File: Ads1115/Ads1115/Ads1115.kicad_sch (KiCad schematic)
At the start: 5 parts, among them U1 ADS1115IDGS

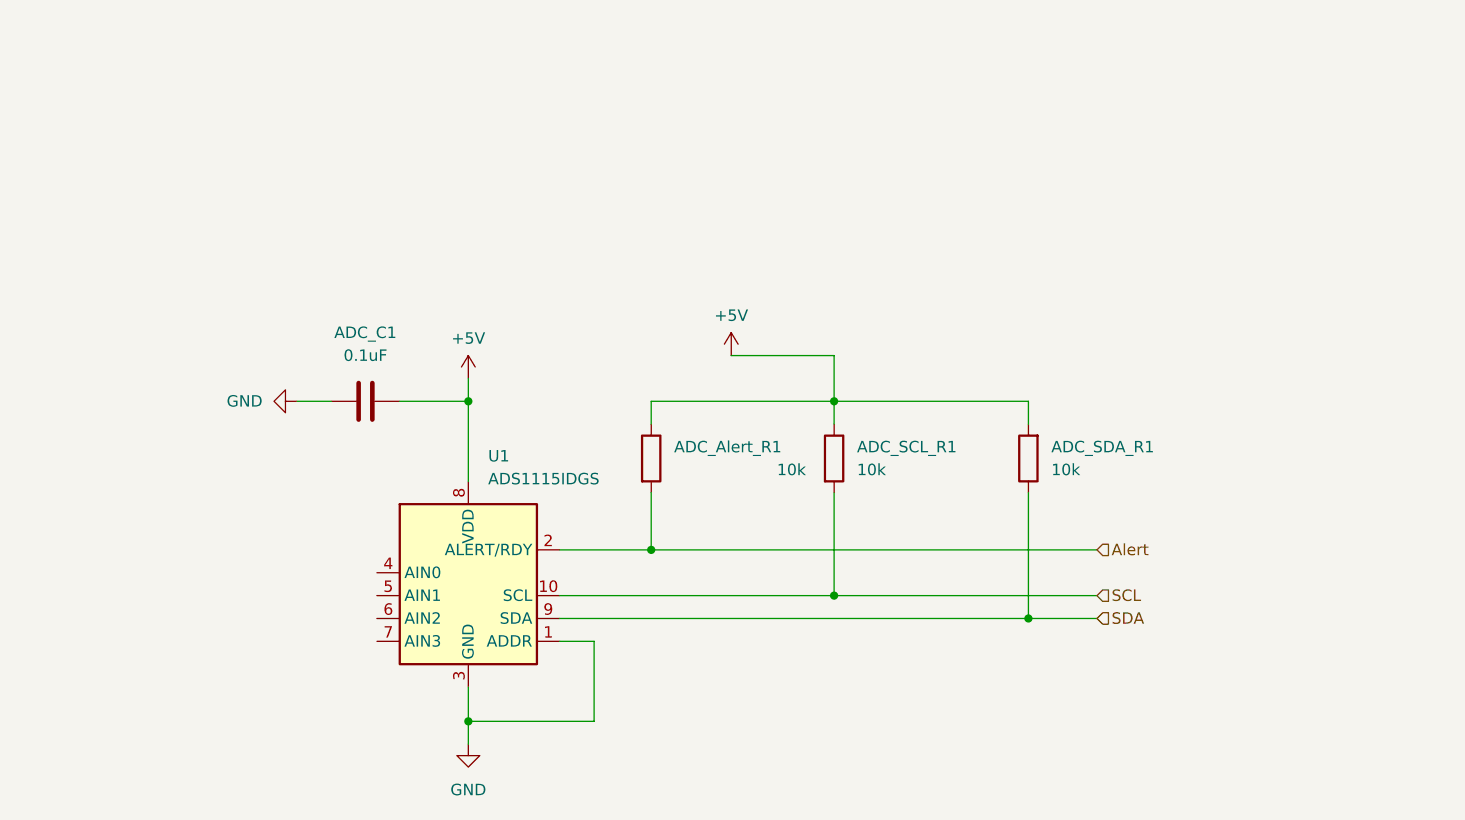
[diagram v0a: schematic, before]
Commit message: updates ads1115 and ads 1248
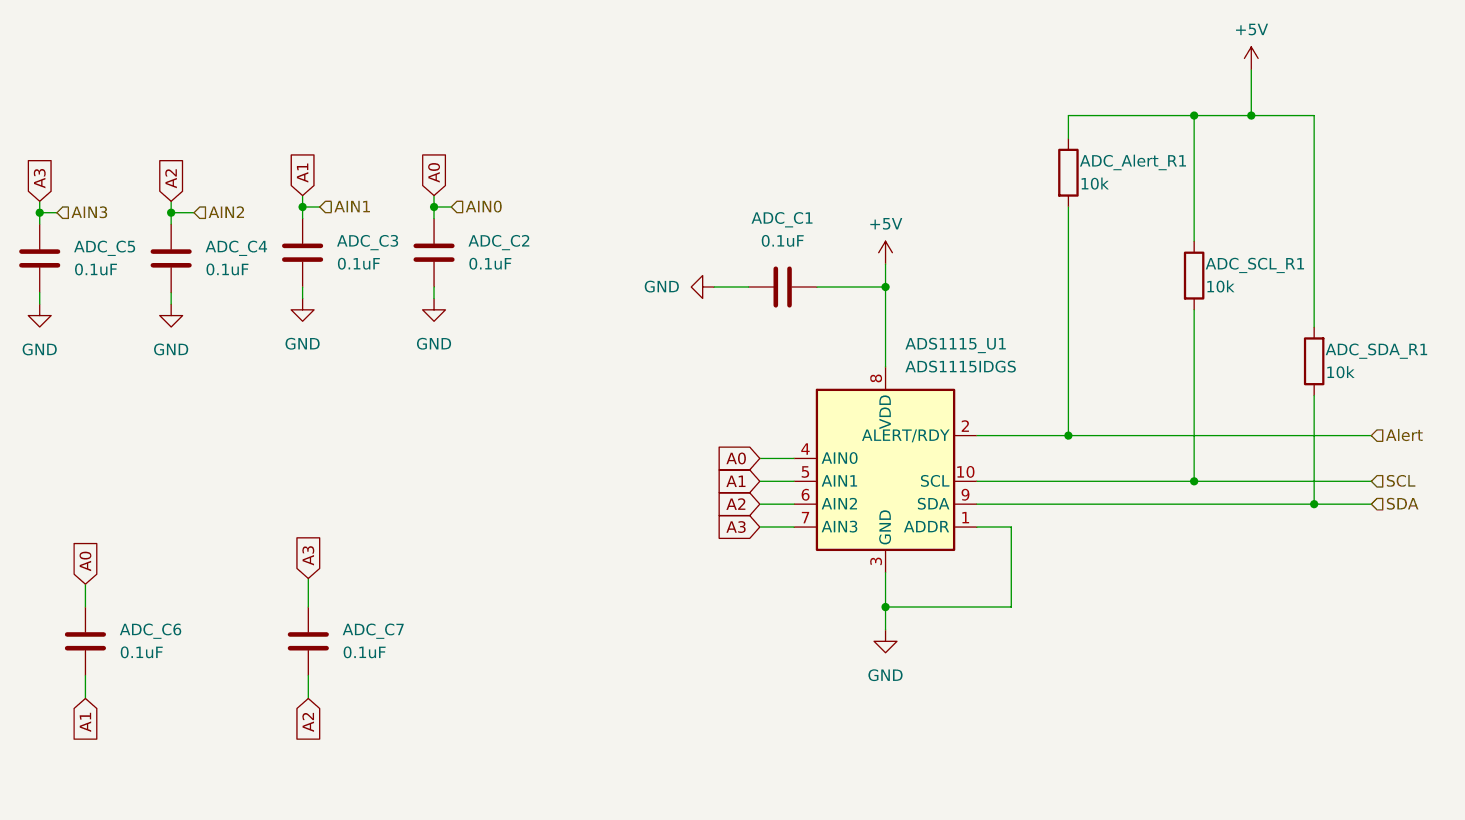
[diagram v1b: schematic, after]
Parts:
- added ADC_C2, ADC_C3, ADC_C4, ADC_C5, ADC_C6, ADC_C7: 0.1uF, Capacitor_SMD:C_0402_1005Metric, symbol Device:C
- renumbered U1 to ADS1115_U1
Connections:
- net GND: now also ADC_C2.1, ADC_C3.1, ADC_C4.1, ADC_C5.1
- net A0: now reaches ADS1115_U1.4 (AIN0)
- net A0: now also ADC_C2.2, ADC_C6.2
- net A1: now reaches ADS1115_U1.5 (AIN1)
- net A1: now also ADC_C3.2, ADC_C6.1
- net A2: now reaches ADS1115_U1.6 (AIN2)
- net A2: now also ADC_C4.2, ADC_C7.1
- net A3: now reaches ADS1115_U1.7 (AIN3)
- net A3: now also ADC_C5.2, ADC_C7.2
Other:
- moved on the sheet: ADC_Alert_R1, ADC_SCL_R1, ADC_SDA_R1, ADS1115_U1
